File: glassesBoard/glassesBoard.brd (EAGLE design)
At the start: 87.4 x 30.9 mm, 131 parts, among them J1 BM10NB(0.8)-16DS-0.4V(51), J2 DF30FC-30DS-0.4V, J3 S2B-XH-A(LF)(SN), J4 GRPB042MWCN-RC, J5 0787324001, J6 FH26W-39S-0.3SHW, J7 105450-0101, U10 ATTINY20-MMH, U11 SN65LVDS822VQFN48, U12 NLAS2750, U13 NX3020NAK, U14 SSM3J338RSOT-23F, U15 NX3020NAK, U16 SSM3J338RSOT-23F, U17 NX3020NAK, U18 2.8, U19 TCR2EF15SOT-25, U2 TPS613222A, U20 MICROSD, U21 MCP73833, U22 FXMA2104UMX, U23 NX3020NAK, U24 FXMA2104UMX, U25 FXMA2104UMX, U26 LM2665M6XSOT23-6, U3 1.8, U4 3.3, U5 SSM3J338RSOT-23F, U6 SSM3J338RSOT-23F, U7 SN65DSI83-Q1S-PQFP-G64, U8 IQS263BDFN10, U9 NX3020NAK

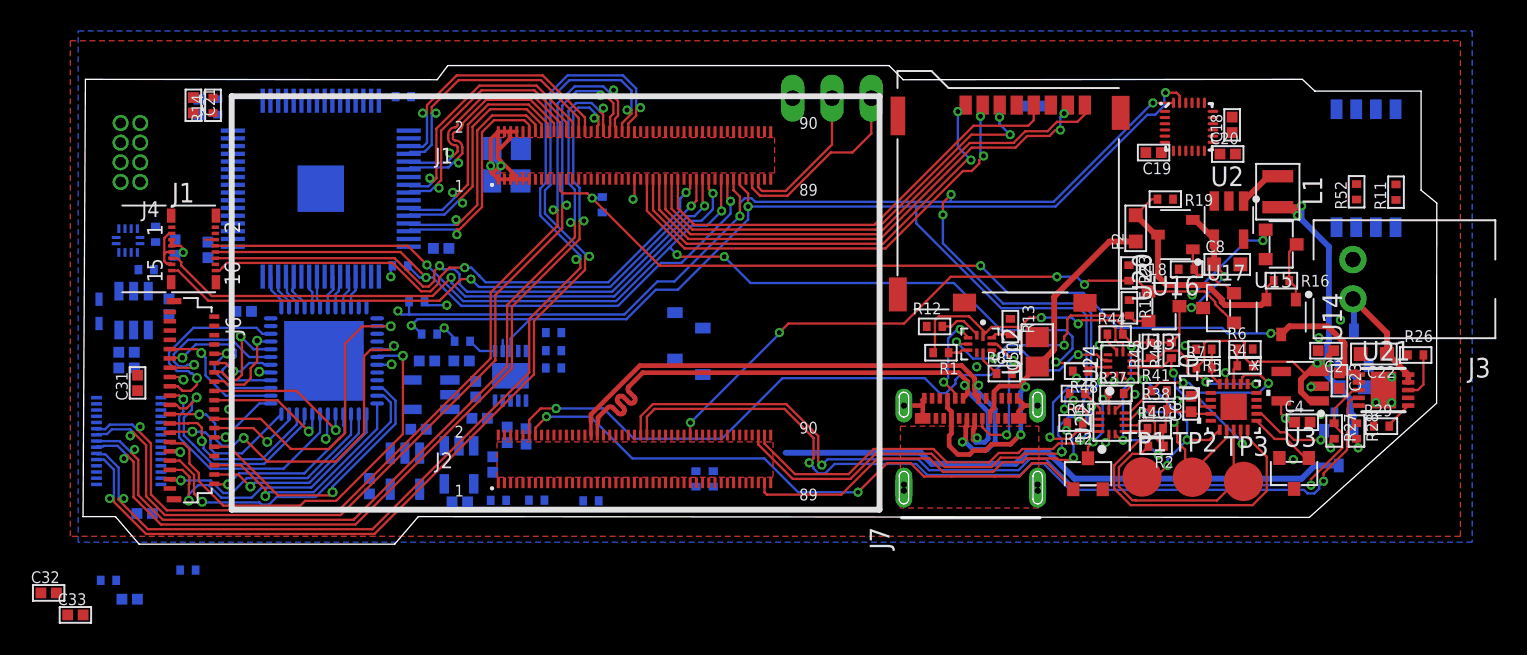
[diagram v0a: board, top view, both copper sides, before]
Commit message: more progress on routing
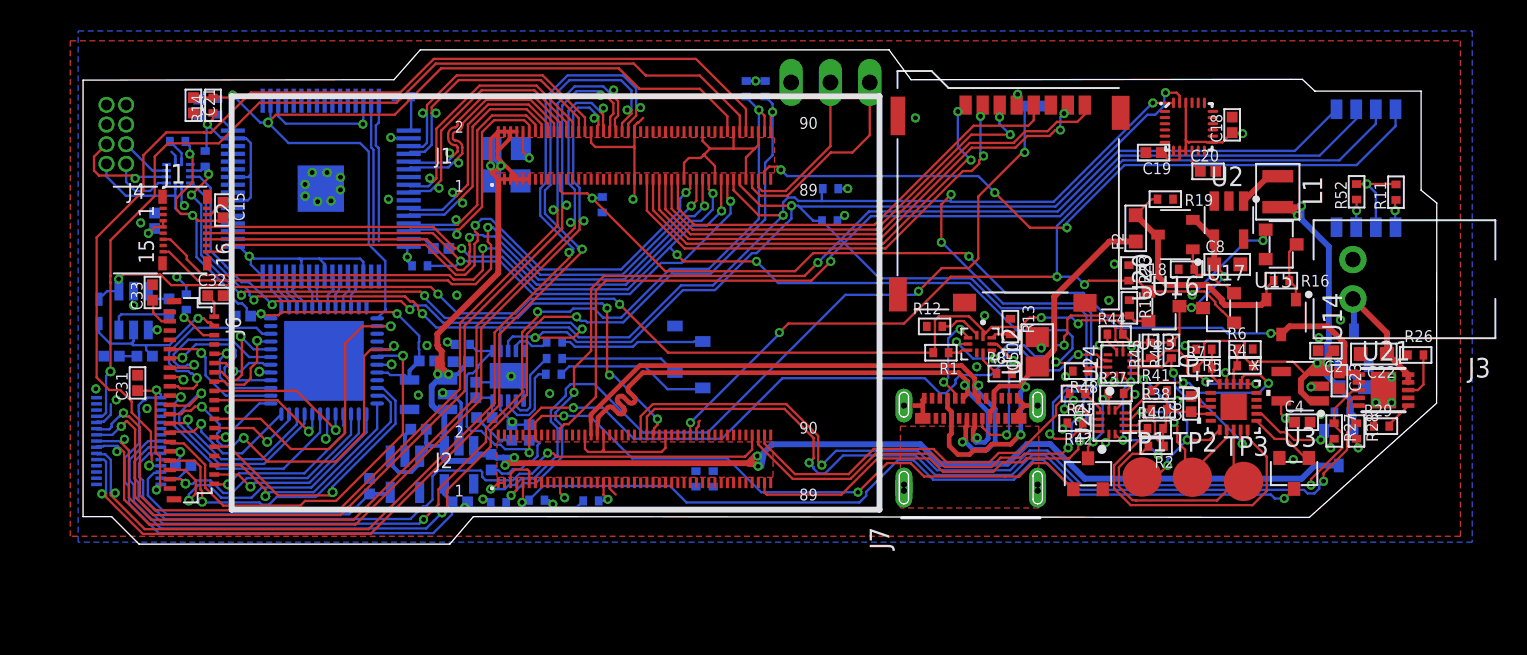
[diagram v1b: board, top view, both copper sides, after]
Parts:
- removed C30: 1uF, thanics-capacitor:C0402
- added R50: 10k, thanics-resistor:R0402
- moved R31 53.0 mm to (43.7, 27.6), turned to 90 degrees
- moved R30 47.6 mm to (42.5, 27.6), turned to 90 degrees
- moved R21 27.7 mm to (48.0, 21.2)
- moved R22 26.9 mm to (47.9, 19.1)
- moved C32 22.0 mm to (8.23, 14.3)
- moved C33 21.4 mm to (4.17, 14.5), turned to 90 degrees
- moved C29 9.30 mm to (6.15, 3.30)
- moved R49 8.11 mm to (7.57, 23.1), turned to 90 degrees
- moved R47 6.16 mm to (5.79, 24.2), turned to 180 degrees
- moved U25 5.41 mm to (5.84, 22.1), turned to 90 degrees
- moved C15 2.75 mm to (8.72, 19.8), flipped to the top, turned to 270 degrees
- moved C14 2.17 mm to (4.30, 19.1)
- moved C20 1.69 mm to (72.3, 22.3)
- moved J4 1.48 mm to (1.83, 24.7)
- moved J1 1.34 mm to (6.26, 18.5)
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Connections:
- removed net !SHUTDOWN_LVDS: U11.37
- removed net LED_B: J4.4, U$1.J2.2, U$1.J2.60
- removed net LED_G: J4.3, U$1.J2.58, U$1.J2.8
- removed net LED_R: J4.5, U$1.J2.6
- removed net SCL: J6.8
- removed net SDA: J6.7
- net +1V5: no longer C30.1
- net +1V8: now also R50.2
- net DSI_EN: now also U$1.J1.76, U11.37; no longer U$1.J2.63
- net GND: no longer C30.2
- net I2C3_SCL: now also J6.8
- net I2C3_SDA: now also J6.7
- net RESETB: now also R50.1
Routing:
- net PM_RESIN_N: track 0.00 -> 70.8 mm, vias 0 -> 3
- net I2C2_SDA: track 0.00 -> 68.6 mm, vias 0 -> 3
- net CAM1_RST: track 0.00 -> 68.3 mm, vias 0 -> 1
- net I2C2_SCL: track 0.00 -> 67.4 mm, vias 0 -> 3
- net BOOT_CONFIG_1: track 0.00 -> 65.0 mm, vias 0 -> 1
- net +1V8: track 17.6 -> 81.1 mm, vias 18 -> 31
- net GND: track 17.5 -> 80.6 mm, vias 15 -> 44
- net CAM1_XCLK: track 0.00 -> 61.3 mm, vias 0 -> 1
- net P$1: track 54.5 -> 114.7 mm, vias 2 -> 8
- net DSI_EN: track 0.00 -> 59.2 mm, vias 0 -> 2
- net +5V: track 55.0 -> 112.9 mm, vias 8 -> 11
- net VREG_L11_SDC: track 0.00 -> 56.7 mm, vias 0 -> 4
- net PHONE_ON_N: track 0.00 -> 55.7 mm, vias 0 -> 2
- net CAM1_PWDN: track 0.00 -> 48.7 mm, vias 0 -> 1
- net FORCED_USB_BOOT: track 0.00 -> 47.2 mm, vias 0 -> 3
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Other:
- board size 87.4 x 30.9 mm -> 87.4 x 31.9 mm
